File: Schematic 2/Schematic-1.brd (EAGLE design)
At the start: 126.3 x 83.1 mm, 37 parts, among them IC1 7805T, IC3 MCP23017SO, Q1 BSS138, Q2 BSS138, U2 LMV358, U3 LMV324

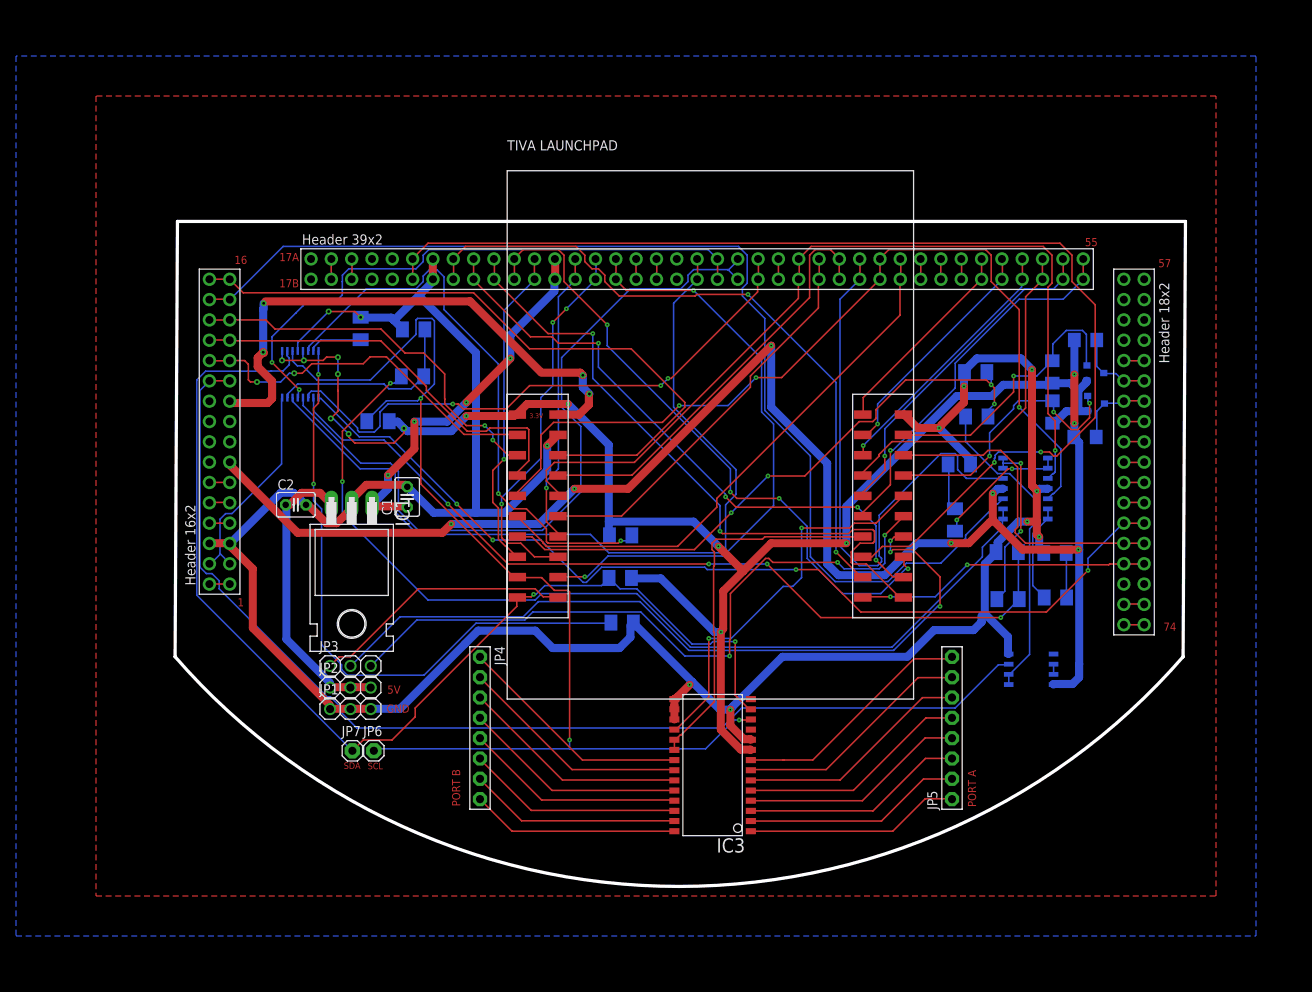
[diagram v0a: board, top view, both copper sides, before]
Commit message: Plugable TIVA changes on 13-06-17
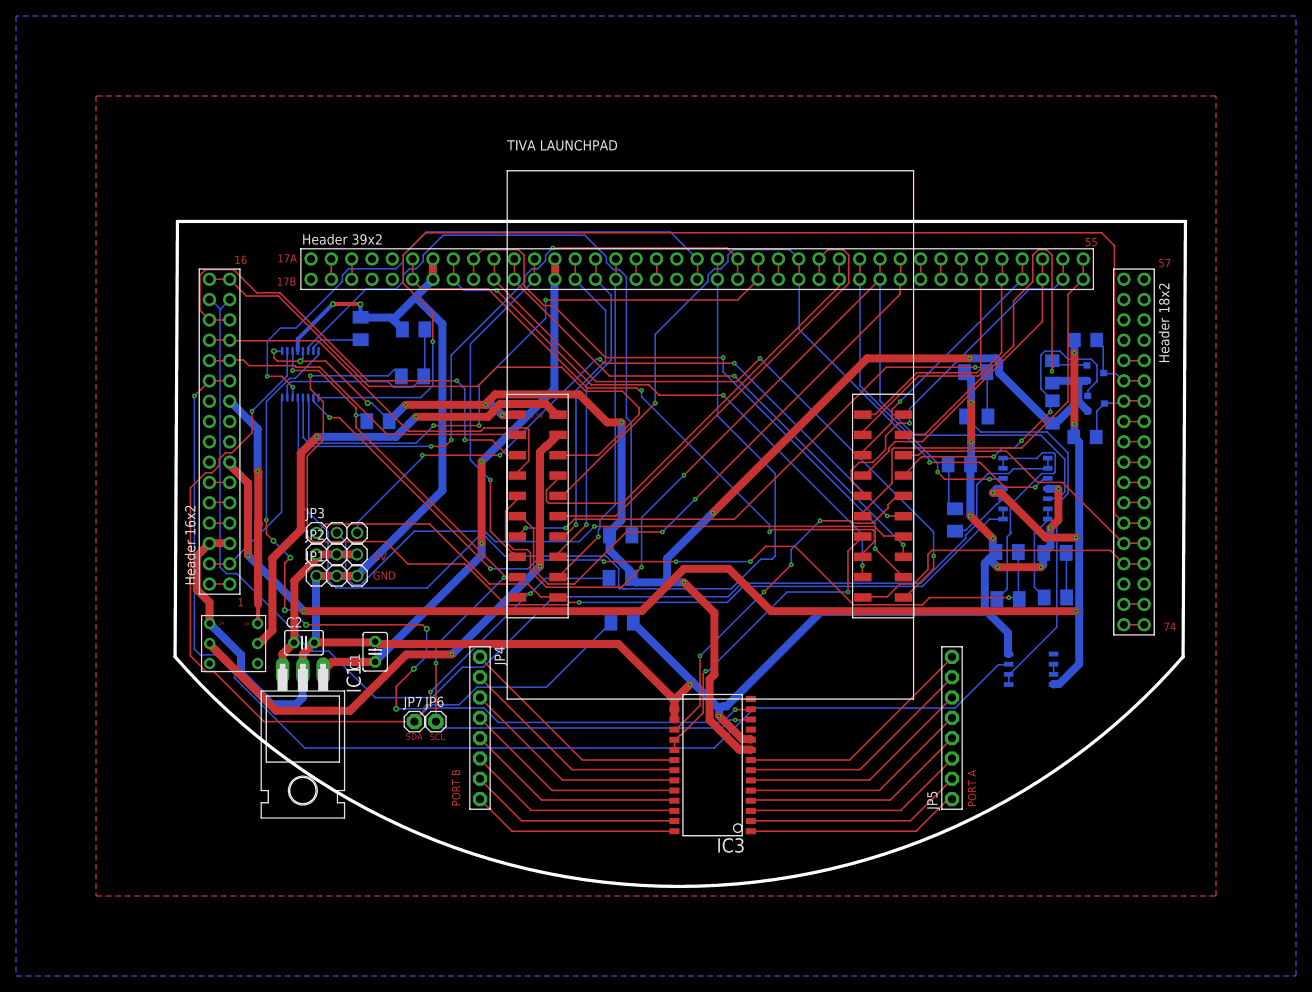
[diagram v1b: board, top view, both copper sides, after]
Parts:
- added U$3: SELF-LOCKING_SWITCHSELF-LOCKING_SWITCH, Switch_Self-locking:SELF-LOCKING_SWITCH
- moved IC1 21.7 mm to (15.9, -12.0)
- moved C1 19.8 mm to (24.9, 0.53)
- moved C2 17.3 mm to (16.0, 1.66)
- moved JP1 16.7 mm to (20.1, 10.0)
- moved JP3 16.7 mm to (20.1, 15.4)
- moved JP2 16.7 mm to (20.1, 12.7)
- moved JP6 8.57 mm to (32.5, -8.20)
- moved JP7 8.57 mm to (29.8, -8.20)
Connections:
- new net 5V2': U$2.VBUS, U$3.2B
- new net GND': U$2.GND, U$3.1B
- net 5V2: now also U$3.2A; no longer U$2.VBUS
- net GND: now also U$3.1A; no longer U$2.GND, U$2.GND'
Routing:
- net GND': track 0.00 -> 69.7 mm, vias 0 -> 2
- net 22: track 145.1 -> 78.4 mm
- net 5V2': track 0.00 -> 61.5 mm, vias 0 -> 2
- net 37: track 74.3 -> 129.3 mm, vias 2 -> 0
- net 5V2: track 71.4 -> 29.5 mm, vias 4 -> 1
- net SCL: track 146.1 -> 106.2 mm, vias 3 -> 5
- net 69: track 121.4 -> 161.2 mm, vias 4 -> 1
- net GND: track 326.3 -> 292.5 mm, vias 11 -> 12
- net 36: track 106.8 -> 73.8 mm, vias 0 -> 2
- net 32: track 74.6 -> 42.8 mm, vias 2 -> 1
- net 44: track 70.3 -> 39.3 mm, vias 0 -> 2
- net N$19: track 78.2 -> 98.6 mm, vias 2 -> 8
- net PB2: track 34.8 -> 54.4 mm
- net 12V: track 47.2 -> 66.8 mm, vias 4 -> 2
- net 5V-SERVO: track 37.2 -> 21.4 mm
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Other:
- board text added: "1A"
- board text added: "2A"
